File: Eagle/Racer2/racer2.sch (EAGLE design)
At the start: 8 parts

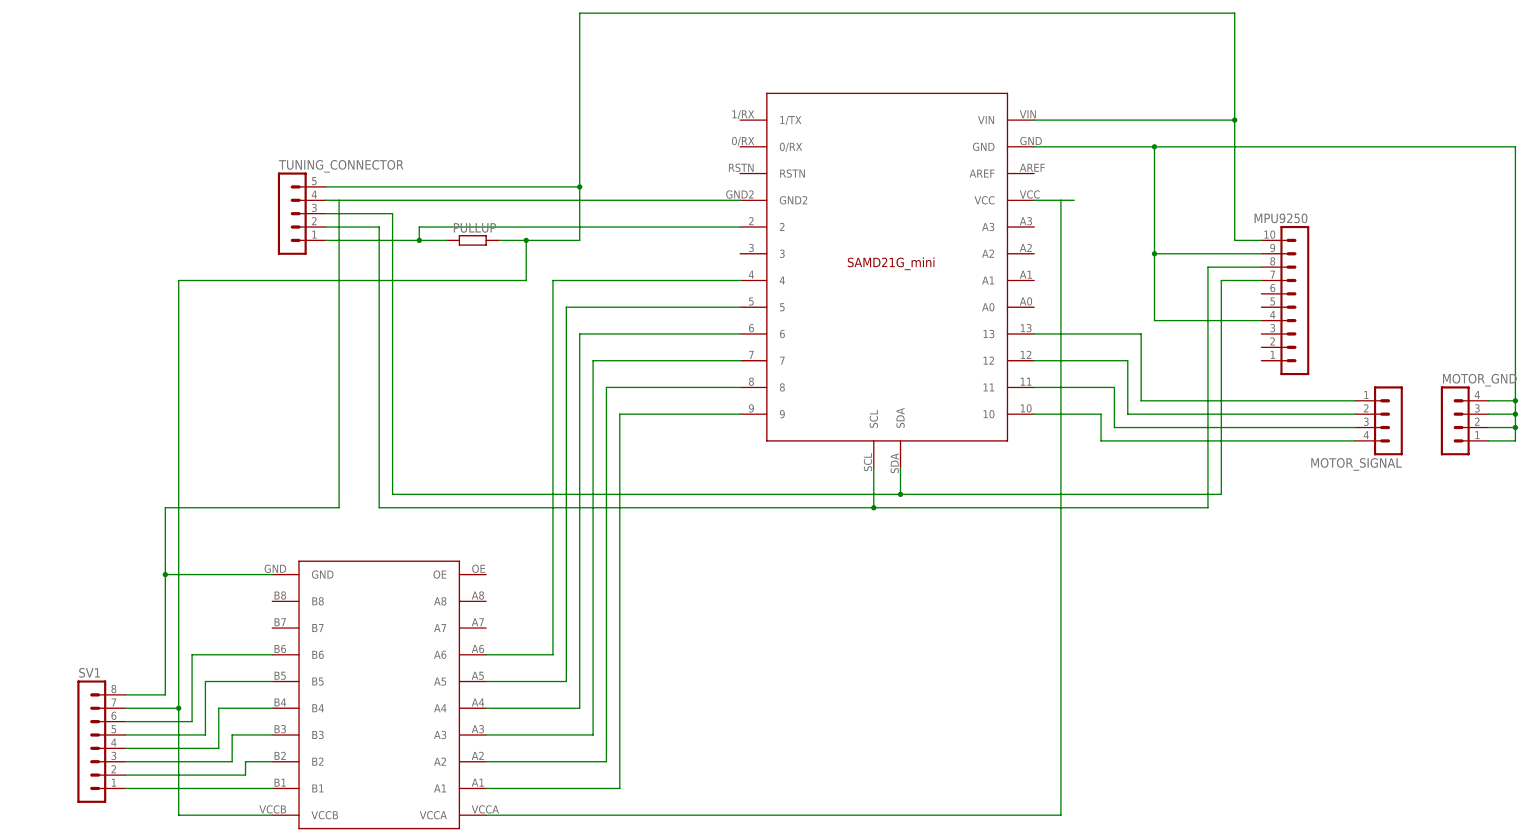
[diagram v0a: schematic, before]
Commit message: Updated.
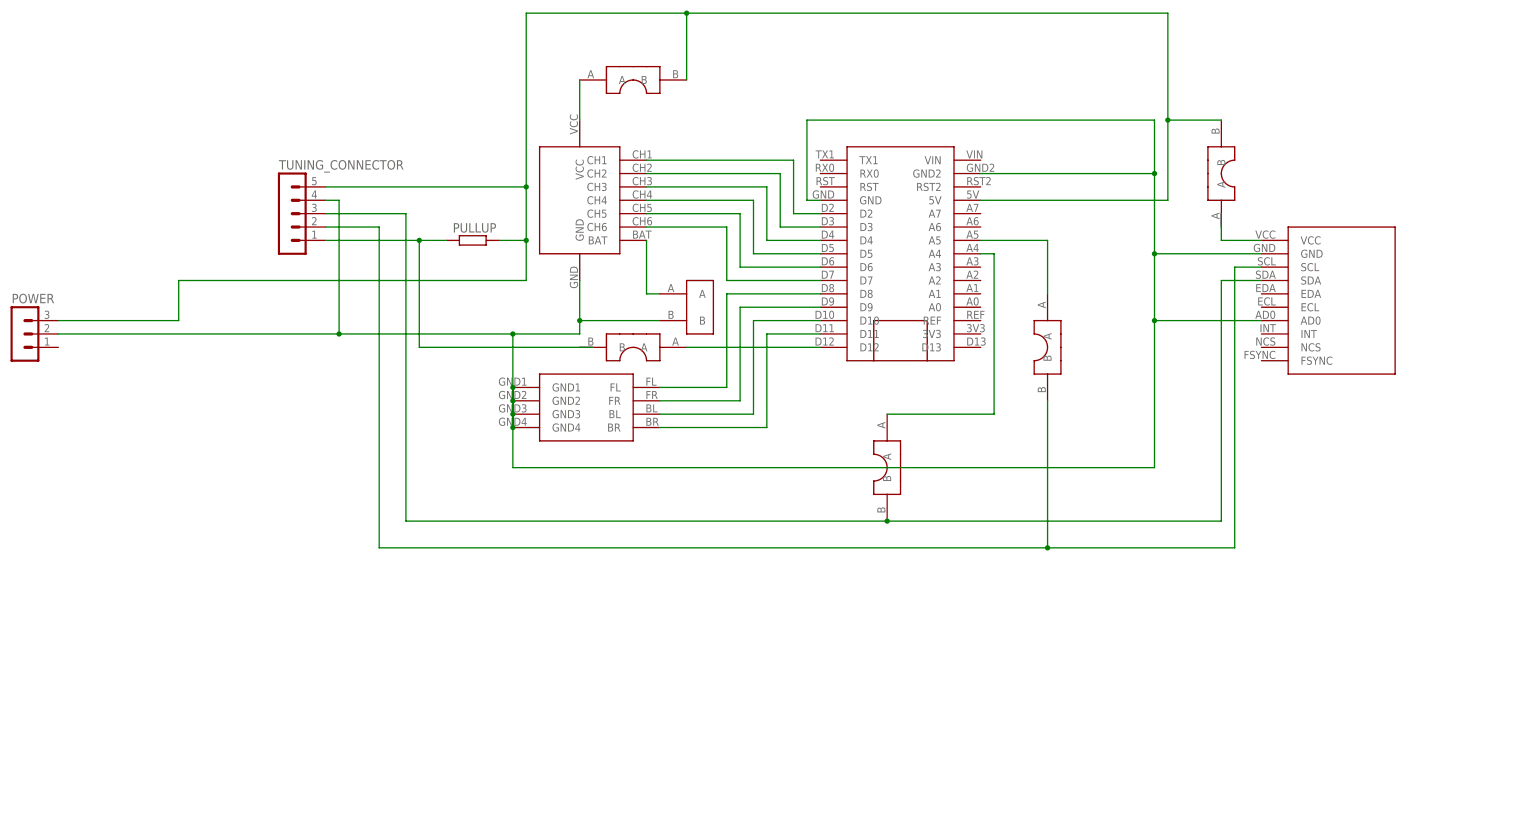
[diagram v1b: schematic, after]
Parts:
- removed MOTOR_GND, MOTOR_SIGNAL: (no value), con-lstb:MA04-1
- removed MPU9250: (no value), con-lstb:MA10-1
- removed SV1: (no value), con-lstb:MA08-1
- added POWER: (no value), con-lstb:MA03-1
- added U$10, U$6, U$7, U$8, U$9: BRIDGE, quadcopter_comp:BRIDGE
- added U$3: FS_RADIO, quadcopter_comp:FS_RADIO
- added U$4: MPU9250, quadcopter_comp:MPU9250
- added U$5: MOTOR_HEADER, quadcopter_comp:MOTOR_HEADER
- U$1: value SAMD21G_MINI -> NANO; device quadcopter_comp:SAMD21G_MINI -> quadcopter_comp:NANO
- U$2: value LEVELSHIFT_8CH -> BUTTON_PULLUP; device quadcopter_comp:LEVELSHIFT_8CH -> quadcopter_comp:BUTTON_PULLUP
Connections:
- removed net GND2: SV1.8, TUNING_CONNECTOR.4, U$1.GND2, U$2.GND
- removed net N$20: U$1.5, U$2.A5
- removed net N$21: U$1.6, U$2.A4
- removed net N$22: U$1.7, U$2.A3
- removed net N$23: U$1.8, U$2.A2
- removed net N$24: U$1.9, U$2.A1
- new net GND: POWER.2, TUNING_CONNECTOR.4, U$1.GND, U$1.GND2, U$2.B, U$3.GND, U$4.AD0, U$4.GND, U$5.GND1, U$5.GND2, U$5.GND3, U$5.GND4
- new net N$15: U$3.VCC, U$9.A
- new net N$17: U$1.A4, U$6.A
- new net N$8: U$1.D6, U$3.CH5
- net 5V: now also POWER.3, U$1.5V, U$10.B, U$9.B; no longer MPU9250.10, SV1.7, U$1.VIN, U$2.VCCB
- net N$1: now also U$1.D12, U$8.A; no longer MPU9250.7, TUNING_CONNECTOR.3, U$1.SDA
- net N$10: now also U$1.D8, U$5.FL; no longer MOTOR_SIGNAL.2, U$1.12
- net N$11: now also U$1.D9, U$5.FR; no longer SV1.4, U$2.B4
- net N$12: now also U$1.D10, U$5.BL; no longer MOTOR_SIGNAL.4, U$1.10
- net N$13: now also U$1.D11, U$5.BR; no longer SV1.5, U$2.B5
- net N$14: now also U$2.A, U$3.BAT; no longer SV1.6, U$2.B6
- net N$16: now also U$8.B; no longer U$1.2
- net N$18: now also TUNING_CONNECTOR.2, U$4.SCL, U$7.B; no longer U$1.VCC, U$2.VCCA
- net N$19: now also U$10.A, U$4.VCC; no longer U$1.4, U$2.A6
- net N$2: now also U$1.A5, U$7.A; no longer MPU9250.8, TUNING_CONNECTOR.2, U$1.SCL
- net N$3: now also TUNING_CONNECTOR.3, U$4.SDA, U$6.B; no longer MOTOR_GND.1, MOTOR_GND.2, MOTOR_GND.3, MOTOR_GND.4, MPU9250.4, MPU9250.9, U$1.GND
- net N$4: now also U$1.D3, U$3.CH2; no longer SV1.1, U$2.B1
- net N$5: now also U$1.D2, U$3.CH1; no longer MOTOR_SIGNAL.3, U$1.11
- net N$6: now also U$1.D4, U$3.CH3; no longer SV1.2, U$2.B2
- net N$7: now also U$1.D5, U$3.CH4; no longer SV1.3, U$2.B3
- net N$9: now also U$1.D7, U$3.CH6; no longer MOTOR_SIGNAL.1, U$1.13
